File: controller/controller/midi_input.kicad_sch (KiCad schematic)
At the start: 7 parts, among them J1-I1 SJ-3524-SMT, U1 H11L1

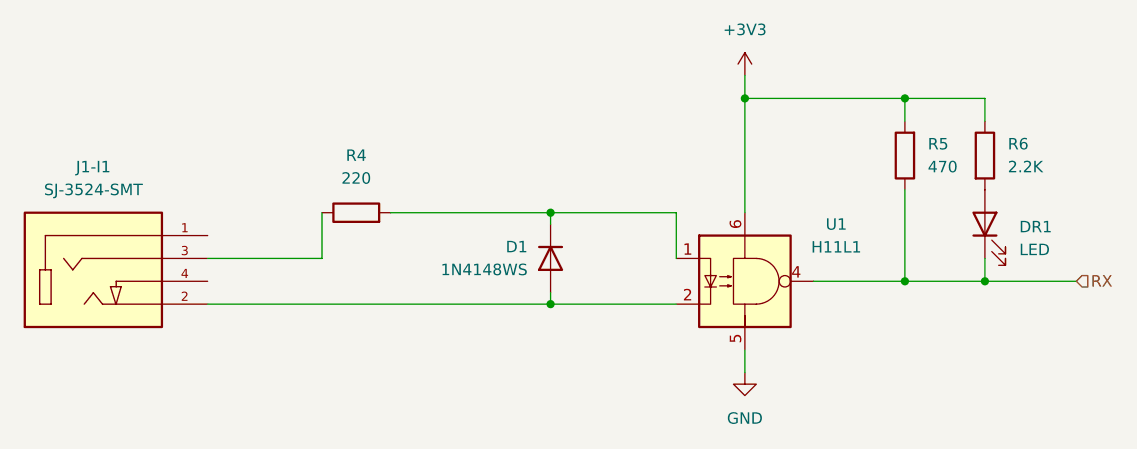
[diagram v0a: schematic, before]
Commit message: prototype 1 sent to production
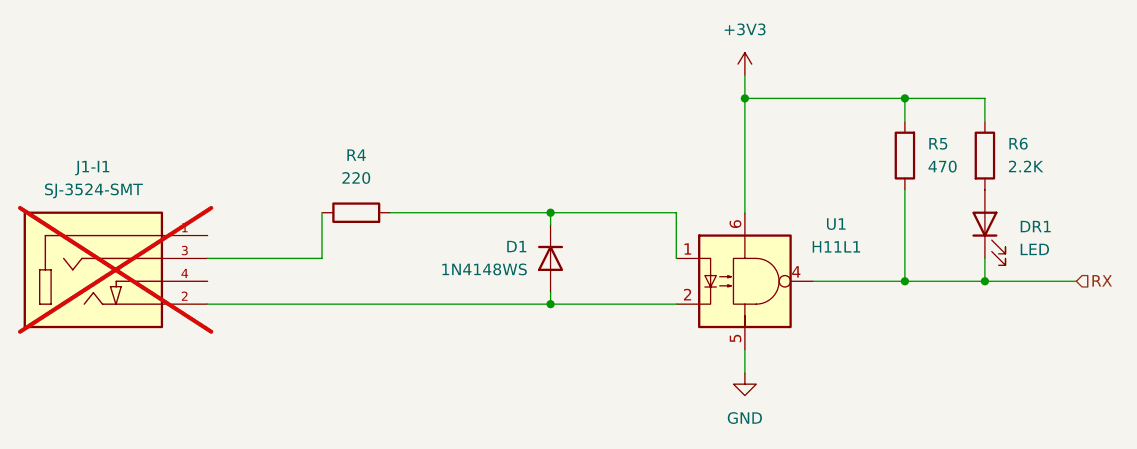
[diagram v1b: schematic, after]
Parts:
- J1-I1: now not fitted
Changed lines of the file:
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@@
 		(in_bom no)
 		(on_board yes)
-		(dnp no)
+		(dnp yes)
 		(property "Reference" "J1-I1"
 			(at 64.77 80.01 0)

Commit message: Merged
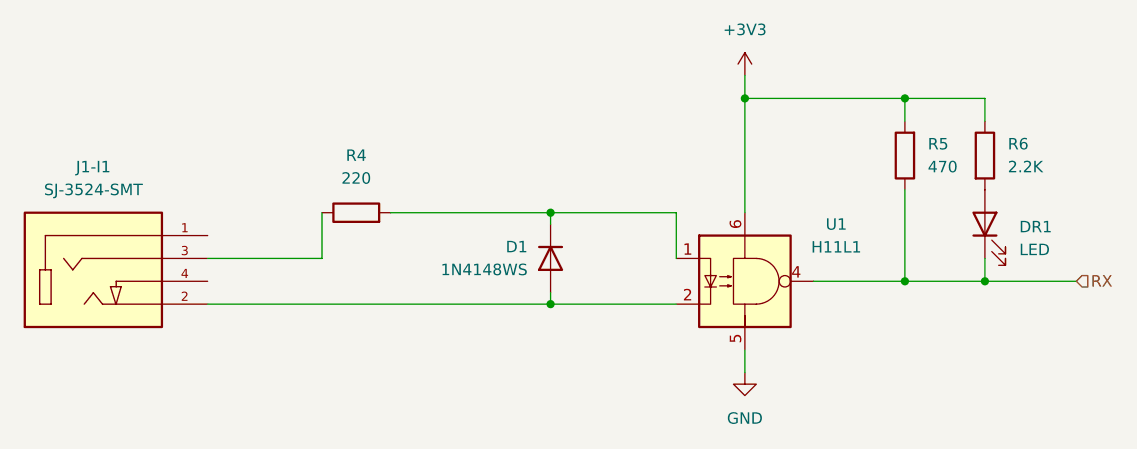
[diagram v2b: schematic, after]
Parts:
- J1-I1: now fitted
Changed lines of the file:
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@@
 		(in_bom no)
 		(on_board yes)
-		(dnp yes)
+		(dnp no)
 		(property "Reference" "J1-I1"
 			(at 64.77 80.01 0)
